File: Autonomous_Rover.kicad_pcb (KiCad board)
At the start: 2 copper layers, 101.6 x 63.5 mm, 42 parts, among them J1 BNO085, J10 BEAM_LIGHT, J11 ESP32_L, J12 ESP32_R, J13 POWER, J2 VL53L5X_L, J3 VL53L5X_M, J4 VL53L5X_R, J5 VEML7700, J6 HC-SR04_M, J7 UART_3V, J8 UART_5V, J9 MOTOR, Q1 AO3400A, Q2 AO3400A, U1 AMS1117-3.3

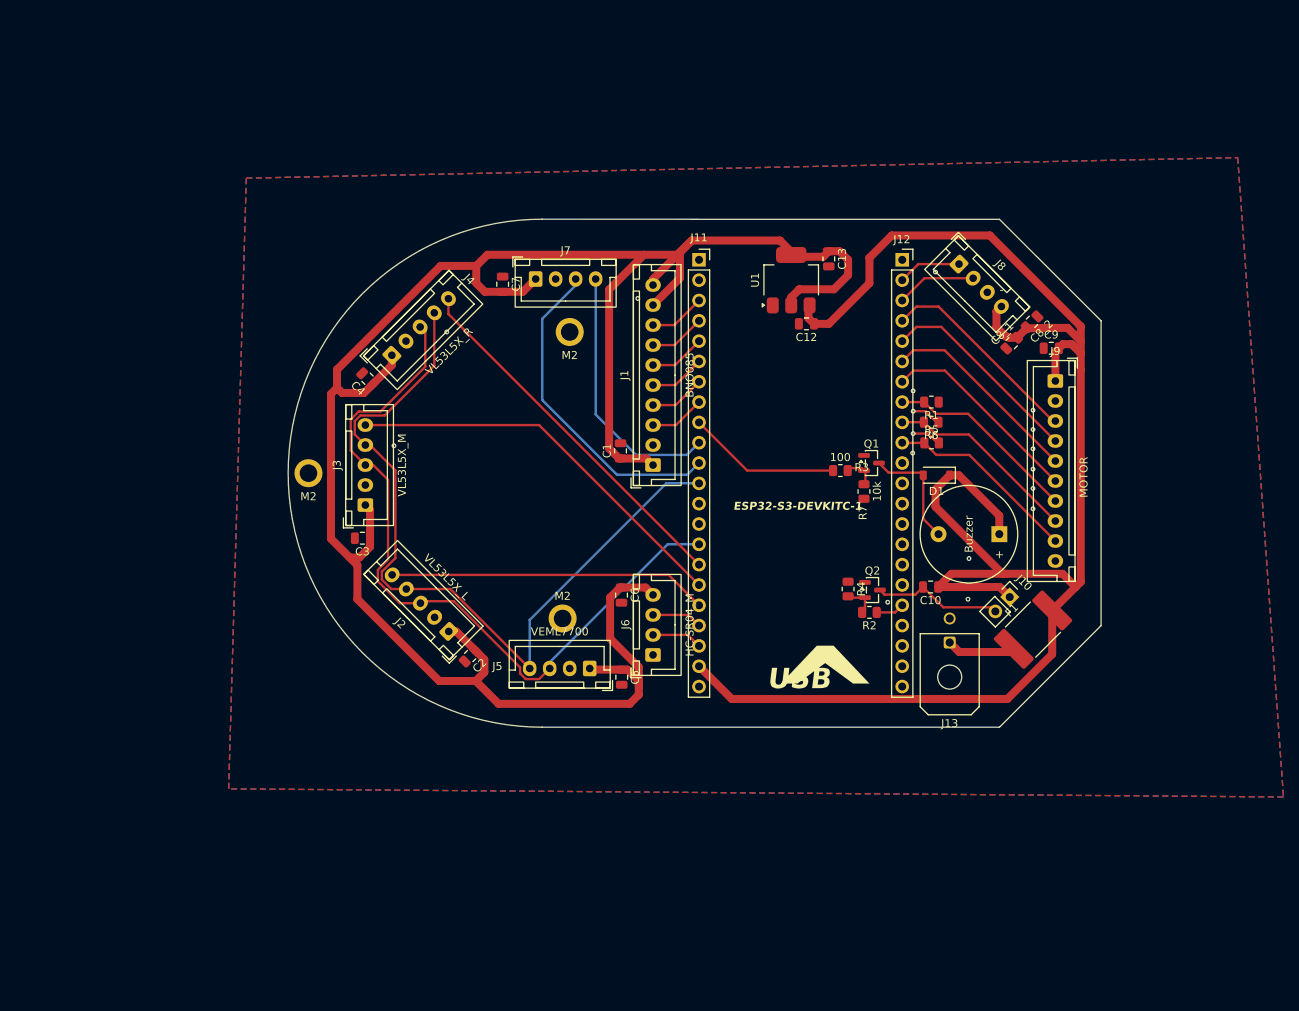
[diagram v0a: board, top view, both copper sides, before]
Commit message: Revision
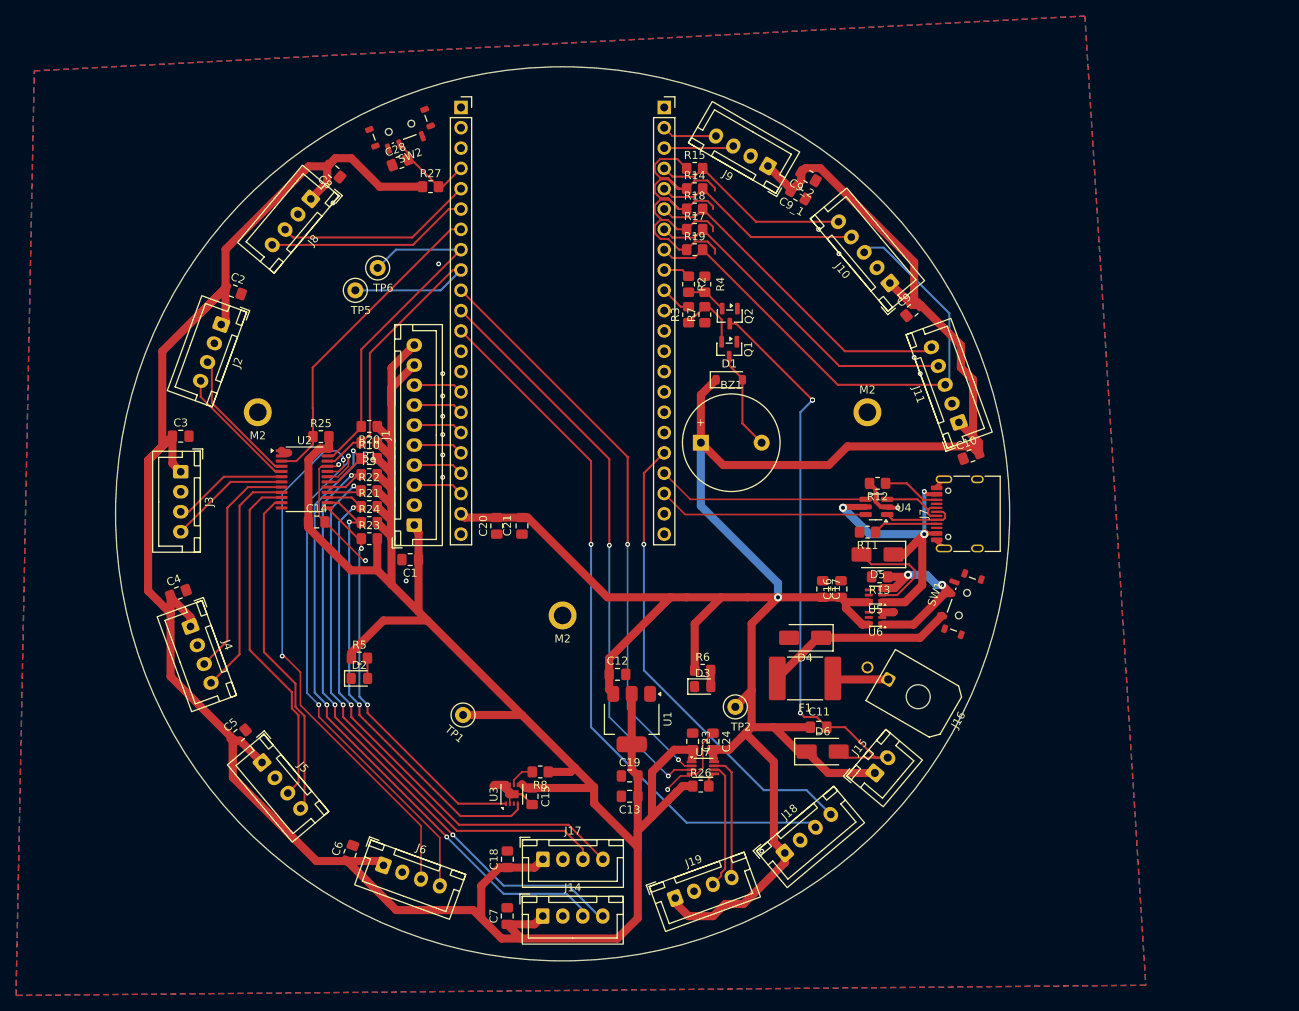
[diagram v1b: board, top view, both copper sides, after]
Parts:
- removed C8_1: 100nF, Capacitor_SMD:C_0805_2012Metric
- removed C8_2: 10uF, Capacitor_SMD:C_0805_2012Metric
- removed the J13 at (188.1, 117.7)
- added C11: 0.1µF, Capacitor_SMD:C_0805_2012Metric_Pad1.18x1.45mm_HandSolder, F.Cu at (171.7, 128.3)
- added C14: 0.1µF, Capacitor_SMD:C_0805_2012Metric_Pad1.18x1.45mm_HandSolder, F.Cu at (109.0, 102.6)
- added C15: 0.1µF, Capacitor_SMD:C_0805_2012Metric_Pad1.18x1.45mm_HandSolder, F.Cu at (135.9, 136.9)
- added C16: 22µF, Capacitor_SMD:C_0805_2012Metric_Pad1.18x1.45mm_HandSolder, F.Cu at (174.5, 111.0)
- added C17: 0.1µF, Capacitor_SMD:C_0805_2012Metric_Pad1.18x1.45mm_HandSolder, F.Cu at (172.2, 111.0)
- added C18: 0.1µF, Capacitor_SMD:C_0805_2012Metric_Pad1.18x1.45mm_HandSolder, F.Cu at (132.8, 144.8)
- added C19: 0.1µF, Capacitor_SMD:C_0805_2012Metric_Pad1.18x1.45mm_HandSolder, F.Cu at (148.1, 134.4)
- added C20: 22µF, Capacitor_SMD:C_0805_2012Metric_Pad1.18x1.45mm_HandSolder, F.Cu at (131.5, 103.1)
- added C21: 0.1µF, Capacitor_SMD:C_0805_2012Metric_Pad1.18x1.45mm_HandSolder, F.Cu at (134.6, 103.1)
- added C23: 0.1µF, Capacitor_SMD:C_0805_2012Metric_Pad1.18x1.45mm_HandSolder, F.Cu at (156.0, 130.0)
- added C24: 0.1µF, Capacitor_SMD:C_0805_2012Metric_Pad1.18x1.45mm_HandSolder, F.Cu at (158.5, 130.0)
- added C28: 0.1µF, Capacitor_SMD:C_0805_2012Metric_Pad1.18x1.45mm_HandSolder, F.Cu at (119.4, 57.7)
- added C8: 0.1µF, Capacitor_SMD:C_0805_2012Metric_Pad1.18x1.45mm_HandSolder, F.Cu at (111.1, 58.8)
- added C9_1: 0.1µF, Capacitor_SMD:C_0805_2012Metric_Pad1.18x1.45mm_HandSolder, F.Cu at (169.2, 61.7)
- added C9_2: 10µF, Capacitor_SMD:C_0805_2012Metric_Pad1.18x1.45mm_HandSolder, F.Cu at (170.4, 59.4)
- added D2: LED, LED_SMD:LED_0805_2012Metric_Pad1.15x1.40mm_HandSolder, F.Cu at (114.3, 122.2)
- added D3: LED, LED_SMD:LED_0805_2012Metric_Pad1.15x1.40mm_HandSolder, F.Cu at (157.2, 123.2)
- added D4: SMAJ5.0A, Diode_SMD:D_SMA, F.Cu at (170.0, 117.1)
- added D5: SMAJ5.0A, Diode_SMD:D_SMA, F.Cu at (179.1, 106.7)
- added D6: SS16, Diode_SMD:D_SMA, F.Cu at (172.2, 131.3)
- added J11: R_MOT, Connector_JST:JST_XH_B5B-XH-A_1x05_P2.50mm_Vertical, F.Cu at (189.2, 90.2)
- added J14: I2C_1, Connector_JST:JST_XH_B4B-XH-A_1x04_P2.50mm_Vertical, F.Cu at (137.2, 151.9)
- added J15: BEAM_LIGHT, Connector_JST:JST_XH_B2B-XH-A_1x02_P2.50mm_Vertical, F.Cu at (178.7, 134.0)
- added J16: POWER, Connector_Molex:Molex_Micro-Fit_3.0_43045-0200_2x01_P3.00mm_Horizontal, F.Cu at (180.4, 122.3)
- added J17: I2C_2, Connector_JST:JST_XH_B4B-XH-A_1x04_P2.50mm_Vertical, F.Cu at (137.2, 144.8)
- added J18: Conn_01x03, Connector_JST:JST_XH_B4B-XH-A_1x04_P2.50mm_Vertical, F.Cu at (167.5, 144.0)
- added J19: Conn_01x03, Connector_JST:JST_XH_B4B-XH-A_1x04_P2.50mm_Vertical, F.Cu at (153.8, 149.6)
- added R10: R, Resistor_SMD:R_0805_2012Metric_Pad1.20x1.40mm_HandSolder, F.Cu at (115.5, 94.7)
- added R11: 5.1kΩ, Resistor_SMD:R_0805_2012Metric_Pad1.20x1.40mm_HandSolder, F.Cu at (177.8, 103.9)
- added R12: 5.1kΩ, Resistor_SMD:R_0805_2012Metric_Pad1.20x1.40mm_HandSolder, F.Cu at (179.1, 97.8)
- added R13: 100kΩ, Resistor_SMD:R_0805_2012Metric_Pad1.20x1.40mm_HandSolder, F.Cu at (179.3, 109.5)
- added R14: 10kΩ, Resistor_SMD:R_0805_2012Metric_Pad1.20x1.40mm_HandSolder, F.Cu at (156.2, 61.0)
- added R15: 10kΩ, Resistor_SMD:R_0805_2012Metric_Pad1.20x1.40mm_HandSolder, F.Cu at (156.2, 58.4)
- added R17: 10kΩ, Resistor_SMD:R_0805_2012Metric_Pad1.20x1.40mm_HandSolder, F.Cu at (156.2, 66.0)
- added R18: 10kΩ, Resistor_SMD:R_0805_2012Metric_Pad1.20x1.40mm_HandSolder, F.Cu at (156.2, 63.5)
- added R19: 10kΩ, Resistor_SMD:R_0805_2012Metric_Pad1.20x1.40mm_HandSolder, F.Cu at (156.2, 68.6)
- added R20: 4.7kΩ, Resistor_SMD:R_0805_2012Metric_Pad1.20x1.40mm_HandSolder, F.Cu at (115.5, 90.7)
- added R21: R, Resistor_SMD:R_0805_2012Metric_Pad1.20x1.40mm_HandSolder, F.Cu at (115.5, 100.7)
- added R22: R, Resistor_SMD:R_0805_2012Metric_Pad1.20x1.40mm_HandSolder, F.Cu at (115.5, 98.7)
- added R23: R, Resistor_SMD:R_0805_2012Metric_Pad1.20x1.40mm_HandSolder, F.Cu at (115.5, 104.7)
- added R24: R, Resistor_SMD:R_0805_2012Metric_Pad1.20x1.40mm_HandSolder, F.Cu at (115.5, 102.7)
- added R25: 10kΩ, Resistor_SMD:R_0805_2012Metric_Pad1.20x1.40mm_HandSolder, F.Cu at (109.5, 91.9)
- added R26: 10kΩ, Resistor_SMD:R_0805_2012Metric_Pad1.20x1.40mm_HandSolder, F.Cu at (157.0, 135.6)
- added R27: 10kΩ, Resistor_SMD:R_0805_2012Metric_Pad1.20x1.40mm_HandSolder, F.Cu at (123.2, 60.7)
- added R8: 10kΩ, Resistor_SMD:R_0805_2012Metric_Pad1.20x1.40mm_HandSolder, F.Cu at (136.9, 133.9)
- added R9: R, Resistor_SMD:R_0805_2012Metric_Pad1.20x1.40mm_HandSolder, F.Cu at (115.5, 96.7)
- added SW1: SW_SPDT, Button_Switch_SMD:SW_SPDT_Shouhan_MSK12C02, F.Cu at (189.7, 112.9)
- added SW2: SW_SPDT, Button_Switch_SMD:SW_SPDT_Shouhan_MSK12C02, F.Cu at (119.4, 53.3)
- added TP1: TestPoint, TestPoint:TestPoint_Loop_D1.80mm_Drill1.0mm_Beaded, F.Cu at (127.3, 126.7)
- added TP2: TestPoint, TestPoint:TestPoint_Loop_D1.80mm_Drill1.0mm_Beaded, F.Cu at (161.3, 125.7)
- added TP5: TestPoint, TestPoint:TestPoint_Loop_D1.80mm_Drill1.0mm_Beaded, F.Cu at (113.8, 73.7)
- added TP6: TestPoint, TestPoint:TestPoint_Loop_D1.80mm_Drill1.0mm_Beaded, F.Cu at (116.6, 70.9)
- added U2: TCA9548APWR, Package_SO:TSSOP-24_4.4x7.8mm_P0.65mm, F.Cu at (107.4, 97.3)
- added U3: SHT31-DIS, Sensor_Humidity:Sensirion_DFN-8-1EP_2.5x2.5mm_P0.5mm_EP1.1x1.7mm, F.Cu at (133.3, 136.7)
- added U4: USBLC6-2SC6, Package_TO_SOT_SMD:SOT-23-6_Handsoldering, F.Cu at (178.9, 100.7)
- added U5: LM66100DCK, Package_TO_SOT_SMD:SOT-363_SC-70-6, F.Cu at (178.8, 111.8)
- added U6: LM66100DCK, Package_TO_SOT_SMD:SOT-363_SC-70-6, F.Cu at (178.8, 114.6)
- added U7: SN74LVC2T45DCUR, Package_SO:VSSOP-8_2.3x2mm_P0.5mm, F.Cu at (157.2, 133.3)
- C1, C2, C3, C4, C5, C6, C7, C9: value 100nF -> 0.1µF; footprint Capacitor_SMD:C_0805_2012Metric -> Capacitor_SMD:C_0805_2012Metric_Pad1.18x1.45mm_HandSolder
- C10: value 10uF -> 0.1µF; footprint Capacitor_SMD:C_0805_2012Metric -> Capacitor_SMD:C_0805_2012Metric_Pad1.18x1.45mm_HandSolder
- C12: footprint Capacitor_SMD:C_0805_2012Metric -> Capacitor_SMD:C_0805_2012Metric_Pad1.18x1.45mm_HandSolder
- C13: value 10uF -> 22µF; footprint Capacitor_SMD:C_0805_2012Metric -> Capacitor_SMD:C_0805_2012Metric_Pad1.18x1.45mm_HandSolder
- F1: footprint Fuse:Fuse_2920_7451Metric -> Fuse:Fuse_2920_7451Metric_Pad2.10x5.45mm_HandSolder
- J10: value BEAM_LIGHT -> L_MOT; footprint Connector_PinHeader_2.54mm:PinHeader_1x02_P2.54mm_Vertical -> Connector_JST:JST_XH_B5B-XH-A_1x05_P2.50mm_Vertical
- J2, J3, J4: footprint Connector_JST:JST_XH_B5B-XH-A_1x05_P2.50mm_Vertical -> Connector_JST:JST_XH_B4B-XH-A_1x04_P2.50mm_Vertical
- J7: value UART_3V -> USB_C_Receptacle_USB2.0_16P; footprint Connector_JST:JST_XH_B4B-XH-A_1x04_P2.50mm_Vertical -> Connector_USB:USB_C_Receptacle_HRO_TYPE-C-31-M-12
- J8: value UART_5V -> UART_3V
- J9: value MOTOR -> UART_5V; footprint Connector_JST:JST_XH_B10B-XH-A_1x10_P2.50mm_Vertical -> Connector_JST:JST_XH_B4B-XH-A_1x04_P2.50mm_Vertical
- R1: value 10k -> 4.7kΩ; footprint Resistor_SMD:R_0805_2012Metric -> Resistor_SMD:R_0805_2012Metric_Pad1.20x1.40mm_HandSolder
- R2, R3: value 100 -> 100Ω; footprint Resistor_SMD:R_0805_2012Metric -> Resistor_SMD:R_0805_2012Metric_Pad1.20x1.40mm_HandSolder
- R4, R7: value 10k -> 10kΩ; footprint Resistor_SMD:R_0805_2012Metric -> Resistor_SMD:R_0805_2012Metric_Pad1.20x1.40mm_HandSolder
- R5: value 1k -> 150Ω; footprint Resistor_SMD:R_0805_2012Metric -> Resistor_SMD:R_0805_2012Metric_Pad1.20x1.40mm_HandSolder
- R6: value 1k -> 300Ω; footprint Resistor_SMD:R_0805_2012Metric -> Resistor_SMD:R_0805_2012Metric_Pad1.20x1.40mm_HandSolder
- moved J8 81.4 mm to (108.2, 62.2), turned to -130 degrees
- moved C7 79.0 mm to (132.8, 151.9), turned to 90 degrees
- moved R5 76.4 mm to (114.3, 119.6)
- moved C13 71.6 mm to (148.1, 136.9), turned to 180 degrees
- moved R1 70.5 mm to (115.5, 92.7)
- moved J7 61.6 mm to (190.5, 101.6), turned to 90 degrees
- moved U1 58.4 mm to (148.3, 127.3), turned to -90 degrees
- moved C2 54.4 mm to (98.5, 73.8), turned to -20 degrees
- moved C12 49.8 mm to (146.6, 121.7), turned to 0 degrees
- moved C5 48.4 mm to (99.3, 129.3), turned to 40 degrees
- moved J2 47.8 mm to (97.0, 77.9), turned to -110 degrees
- moved R2 46.8 mm to (155.4, 72.9), turned to -90 degrees
- moved C6 46.8 mm to (113.1, 144.0), turned to 70 degrees
- moved H3 46.0 mm to (177.8, 88.9)
- moved J9 44.9 mm to (165.4, 58.1), turned to 150 degrees
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- renumbered J11 to J12, J12 to J13
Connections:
- C10 pad 1: +5V -> GND
- C10 pad 2: Net-(J10-Pin_2) -> +5V
- C7 pad 1: GND -> +3V3
- C7 pad 2: +3V3 -> GND
- F1 pad 2: +5V -> /POWER/PWR_IN
- J1 pad 3: /GPIO8 -> INT
- J1 pad 4: /GPIO7 -> MISO
- J1 pad 5: /GPIO6 -> SPICLK
- J1 pad 6: /CS -> MOSI
- J1 pad 7: /INT -> CS0
- J1 pad 8: /RST -> SPI_RST
- J10 pad 2: Net-(J10-Pin_2) -> GND
- J12 pad 10: /UART1_TX -> LED1
- J12 pad 11: /UART1_RX -> LED2
- J12 pad 12: SDA -> SER_PWM1
- J12 pad 15: SCL -> SPI_RST
- J12 pad 16: /LPN_R -> CS0
- J12 pad 17: /LPN_M -> MOSI
- J12 pad 18: /LPN_L -> SPICLK
- J12 pad 19: /TRIG -> MISO
- J12 pad 20: /ECHO -> INT
- J12 pad 3: /RST -> unconnected-(J12-Pin_3-Pad3)
- J12 pad 4: /INT -> MODE_SW
- J12 pad 5: /CS -> UART1_TX
- J12 pad 6: /GPIO6 -> UART1_RX
- J12 pad 7: /GPIO7 -> IIC_RST
- J12 pad 8: /GPIO8 -> SDA
- J12 pad 9: /BUZZ_PWM -> SCL
- J13 pad 10: /R_IS -> BUZZ_PWM
- J13 pad 18: /LIGHT_PWM -> SER_PWM2
- J13 pad 19: unconnected-(J12-Pin_19-Pad19) -> D+
- J13 pad 2: /UART0_TX -> UART0_TX
- J13 pad 20: unconnected-(J12-Pin_20-Pad20) -> D-
- J13 pad 3: /UART0_RX -> UART0_RX
- J13 pad 4: /L_RPWM -> L_LPWM
- J13 pad 5: /L_LPWM -> L_RPWM
- J13 pad 6: /R_RPWM -> R_LPWM
- J13 pad 7: /R_LPWM -> R_RPWM
- J13 pad 8: /MOT_EN -> MOT_EN
- J13 pad 9: /L_IS -> LIGHT_PWM
- J2 pad 3: SCL -> /INPUT/SD_0
- J2 pad 4: SDA -> /INPUT/SC_0
- J3 pad 3: SCL -> /INPUT/SD_1
- J3 pad 4: SDA -> /INPUT/SC_1
- J4 pad 3: SCL -> /INPUT/SD_2
- J4 pad 4: SDA -> /INPUT/SC_2
- J5 pad 3: SCL -> /INPUT/SD_3
- J5 pad 4: SDA -> /INPUT/SC_3
- J6 pad 1: GND -> +3V3
- J6 pad 2: /ECHO -> GND
- J6 pad 3: /TRIG -> /INPUT/SC_7
- J6 pad 4: +3V3 -> /INPUT/SD_7
- J8 pad 1: /UART0_TX -> +3V3
- J8 pad 2: /UART0_RX -> GND
- J8 pad 3: GND -> UART1_TX
- J8 pad 4: +5V -> UART1_RX
- J9 pad 3: /L_RPWM -> UART0_RX
- J9 pad 4: /L_LPWM -> UART0_TX
- Q2 pad 3: Net-(J10-Pin_2) -> Net-(D6-A)
- R1 pad 1: GND -> +3V3
- R1 pad 2: /MOT_EN -> SCL
- R2 pad 1: /LIGHT_PWM -> LIGHT_PWM
- R3 pad 1: /BUZZ_PWM -> Net-(Q1-G)
- R3 pad 2: Net-(Q1-G) -> BUZZ_PWM
- R5 pad 1: /R_IS -> +3V3
- R5 pad 2: GND -> Net-(D2-A)
- R6 pad 1: GND -> +5V
- R6 pad 2: /L_IS -> Net-(D3-A)
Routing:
- net +3V3: track 268.4 -> 456.1 mm
- net GND: track 7.45 -> 116.9 mm, vias 17 -> 18
- net SER_PWM1: track 0.00 -> 89.5 mm, vias 0 -> 1
- net +5V: track 216.3 -> 304.3 mm, vias 0 -> 1
- net /INPUT/SC_6: track 0.00 -> 85.5 mm, vias 0 -> 3
- net /INPUT/SD_6: track 0.00 -> 82.2 mm, vias 0 -> 3
- net /INPUT/SC_5: track 0.00 -> 74.2 mm, vias 0 -> 2
- net Net-(D6-A): track 0.00 -> 73.7 mm, vias 0 -> 3
- net LED2: track 0.00 -> 72.1 mm, vias 0 -> 2
- net /INPUT/SD_5: track 0.00 -> 72.1 mm, vias 0 -> 2
- net LED1: track 0.00 -> 71.9 mm, vias 0 -> 2
- net /INPUT/SC_7: track 0.00 -> 69.2 mm, vias 0 -> 2
- net /INPUT/SD_7: track 0.00 -> 67.2 mm, vias 0 -> 2
- net MOT_EN: track 0.00 -> 66.4 mm
- net SER_PWM2: track 0.00 -> 59.1 mm, vias 0 -> 1
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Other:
- board size 101.6 x 63.5 mm -> 111.8 x 111.8 mm
- board text removed: "-"
- board text removed: "ESP32-S3-DEVKITC-1"
- board text removed: "USB"
- board text removed: "^"
